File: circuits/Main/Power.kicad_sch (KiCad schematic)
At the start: 55 parts, among them IC1 DCDC_MPM3620A, J1 Conn_01x02_Male, J10 Conn_01x02_Male, J11 Conn_01x02_Male, J12 Conn_01x02_Male, J13 Conn_01x02_Male, J14 Conn_01x02_Male, J15 Conn_01x02_Male, J9 Conn_01x02_Male, Q1 DI035P04PT, Q2 BSS138, Q3 SSM3J332R, Q4 BSS138, Q5 DI035P04PT, SW1 SW_SPDT_White, U1 AZ1117CH-3.3

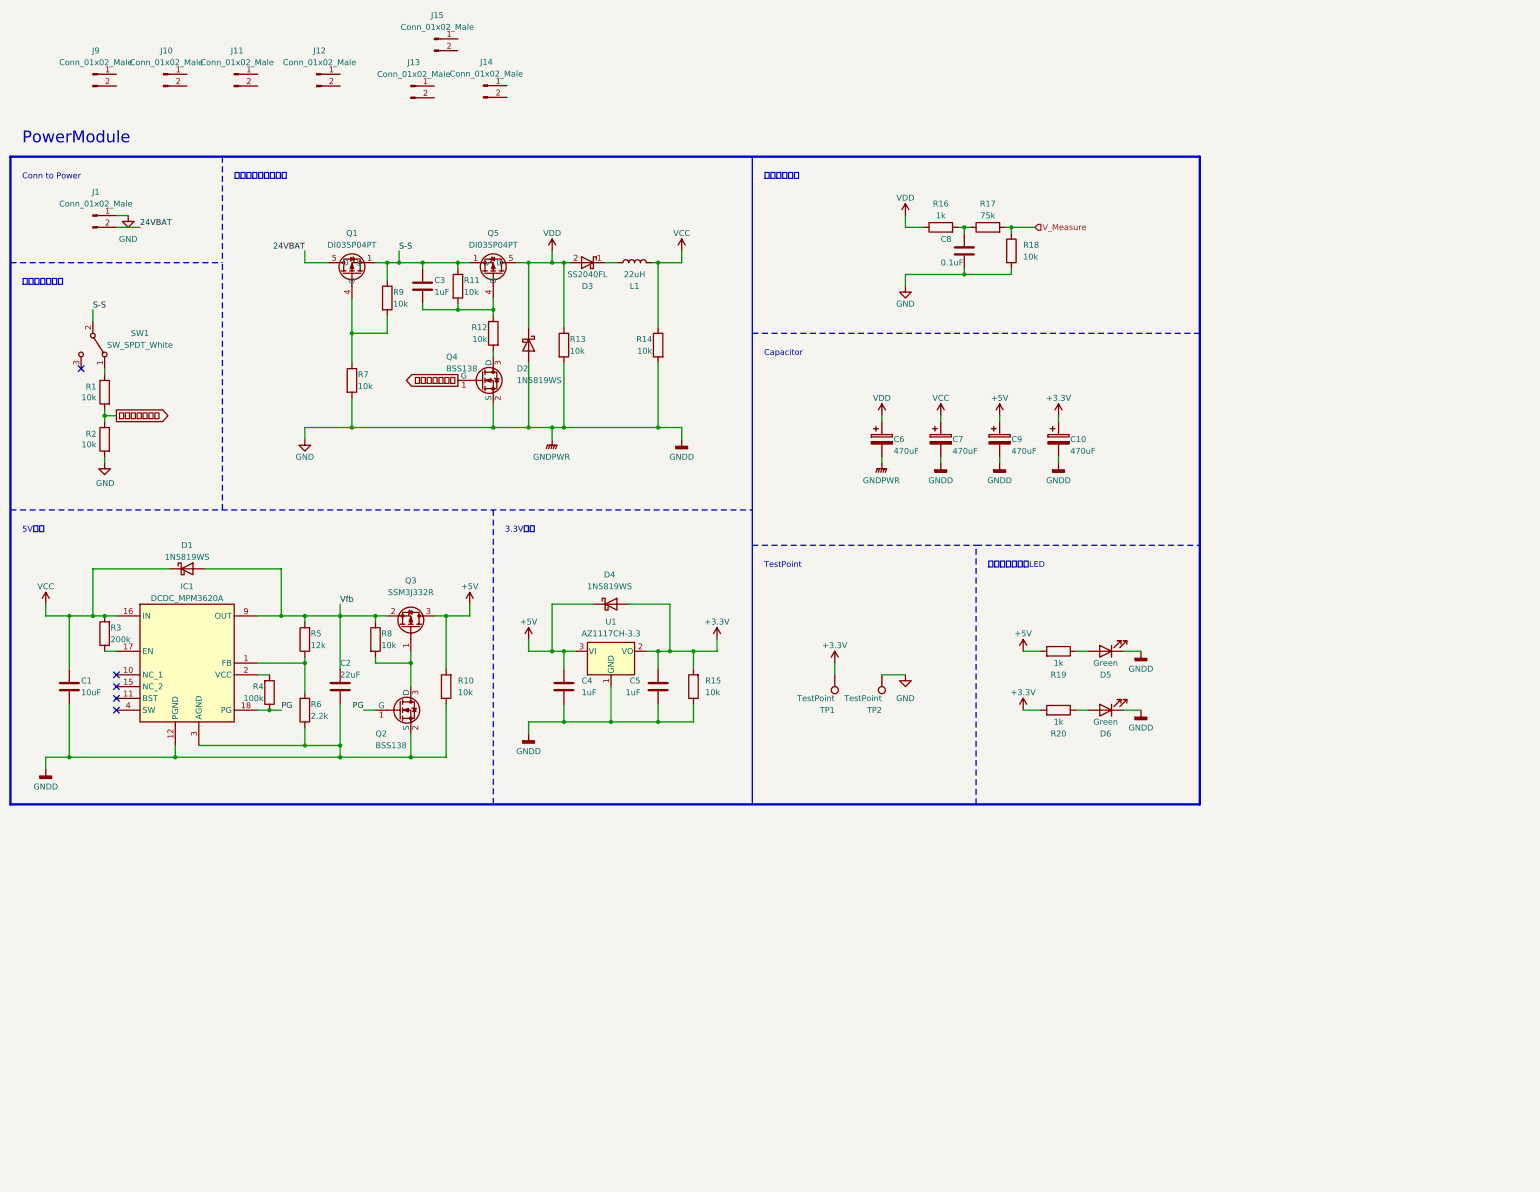
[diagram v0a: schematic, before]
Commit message: こみっと
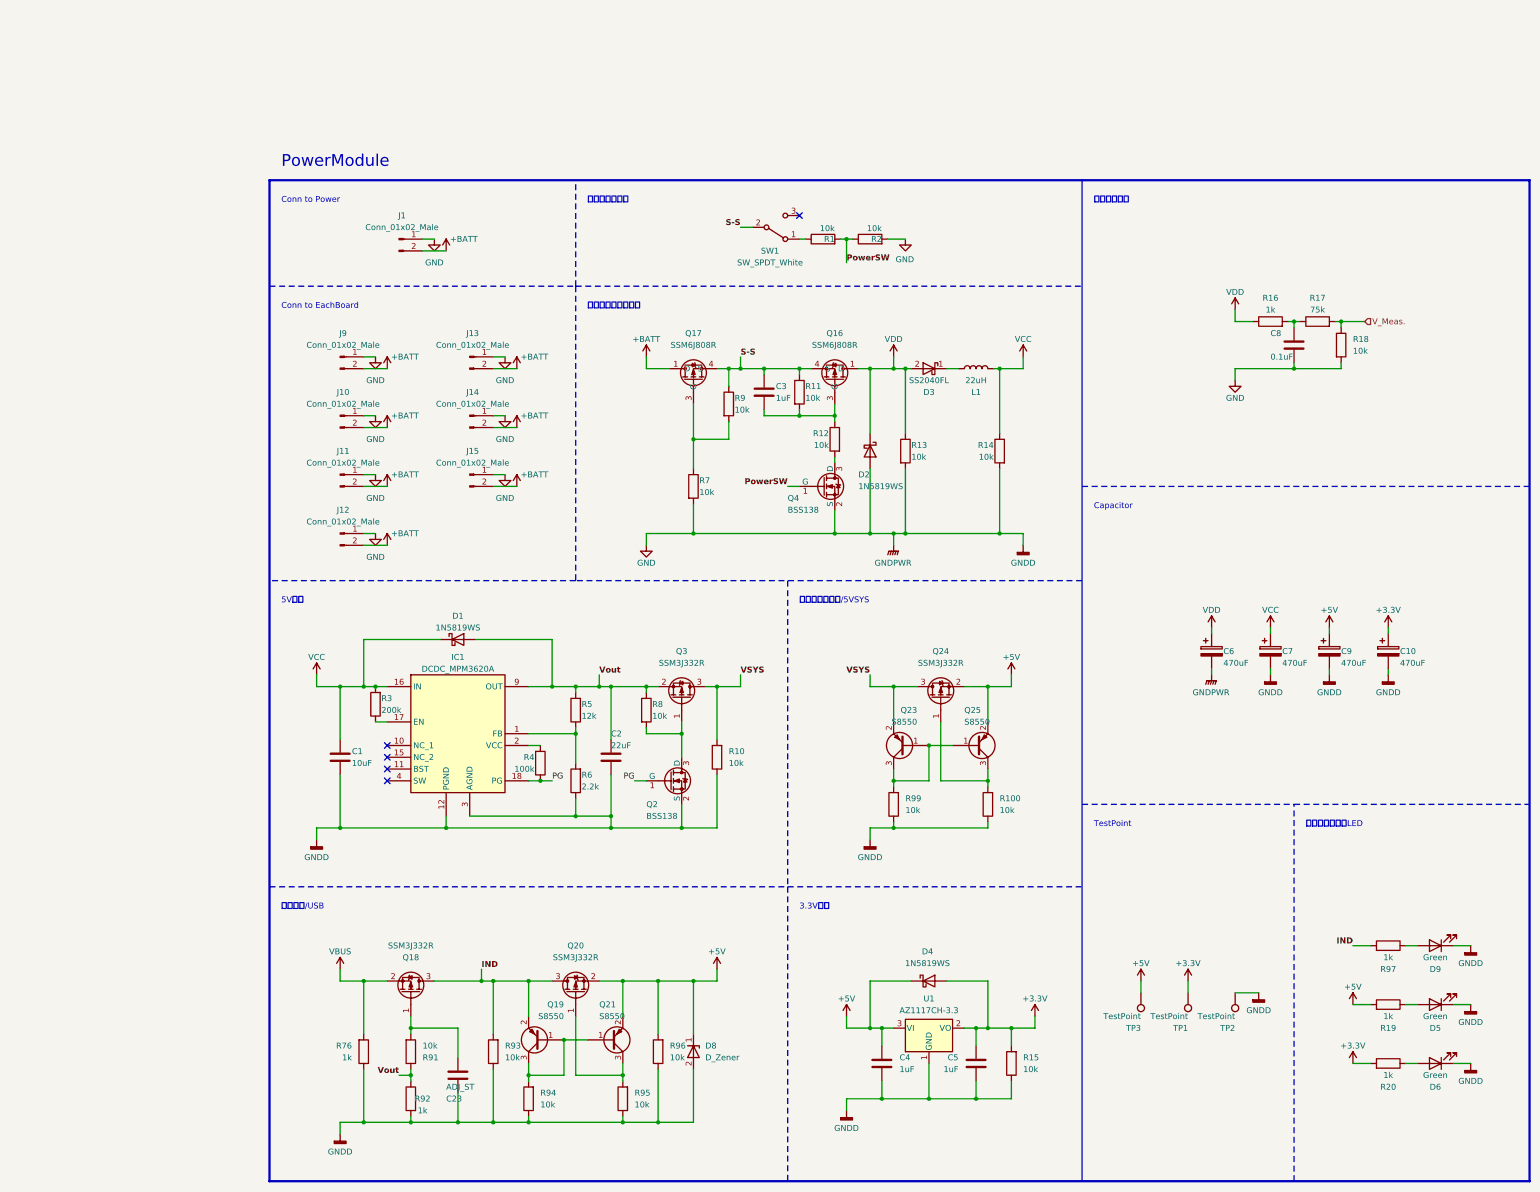
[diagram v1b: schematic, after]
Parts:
- removed Q1, Q5: DI035P04PT, MyLibrary:Package_TSON-Advance, symbol Transistor_FET:AON6411
- added C23: ADJ_ST, Capacitor_SMD:C_0603_1608Metric, symbol Device:C
- added D8: D_Zener, Diode_SMD:D_SOD-323_HandSoldering, symbol Device:D_Zener
- added D9: Green, LED_SMD:LED_0603_1608Metric_Pad1.05x0.95mm_HandSolder, symbol Device:LED
- added Q16, Q17: SSM6J808R, MyLibrary:Package_TSOP6F, symbol Transistor_FET:PMN48XP
- added Q18, Q20, Q24: SSM3J332R, Package_TO_SOT_SMD:SOT-23W, symbol Device:Q_PMOS_GSD
- added Q19, Q21, Q23, Q25: S8550, Package_TO_SOT_SMD:SOT-23, symbol Device:Q_PNP_BEC
- added R100, R91, R93, R94, R95, R96, R99: 10k, Resistor_SMD:R_0402_1005Metric, symbol Device:R
- added R76, R92, R97: 1k, Resistor_SMD:R_0402_1005Metric, symbol Device:R
- added TP3: TestPoint, TestPoint:TestPoint_THTPad_D2.0mm_Drill1.0mm, symbol Connector:TestPoint
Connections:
- net 24VBAT is gone; now on net +BATT: J1.2 (Pin_2)
- net +5V: now also D8.1 (K), Q20.2 (S), Q21.2 (E), Q24.2 (S), Q25.2 (E), R96.2, TP3.1; no longer Q3.3 (D), R10.2
- net GND: now also J10.1 (Pin_1), J11.1 (Pin_1), J12.1 (Pin_1), J13.1 (Pin_1), J14.1 (Pin_1), J15.1 (Pin_1), J9.1 (Pin_1), C23.1, D8.2 (A), D9.1 (K), R100.1, R76.1, R92.2, R93.1, R94.1, R95.1, R96.1, R99.1
- net S-S: now also Q16.4 (S), Q17.4 (S)
- net VDD: now also Q16.1 (D), Q16.2 (D), Q16.5 (D), Q16.6 (D)
- net at R7.1, R9.2: now also Q17.3 (G)
- net at C3.2, R11.2, R12.1: now also Q16.3 (G)
- net +BATT: now reaches J15.2 (Pin_2)
- net +BATT: now also J10.2 (Pin_2), J11.2 (Pin_2), J12.2 (Pin_2), J13.2 (Pin_2), J14.2 (Pin_2), J9.2 (Pin_2), Q17.1 (D), Q17.2 (D), Q17.5 (D), Q17.6 (D)
- net V_Measure renamed V_Meas.
- net Vfb renamed Vout
- net Vout: now also R91.1, R92.1
- net 主電源スイッチ renamed PowerSW
- new net: D9.2 (A), R97.1
- new net: Q19.1 (B), Q19.3 (C), Q21.1 (B), R94.2
- new net: Q23.1 (B), Q23.3 (C), Q25.1 (B), R99.2
- new net: C23.2, Q18.1 (G), R91.2
- new net: Q24.1 (G), Q25.3 (C), R100.2
- new net: Q20.1 (G), Q21.3 (C), R95.2
- new net IND: Q18.3 (D), Q19.2 (E), Q20.3 (D), R93.2, R97.2
- new net VBUS: Q18.2 (S), R76.2
- new net VSYS: Q23.2 (E), Q24.3 (D), Q3.3 (D), R10.2
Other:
- note added: "Conn to EachBoard"
- note added: "理想ダイオード/5VSYS"
- note added: "電源切替/USB"
- moved on the sheet: C1, C10, C2, C3, C4, C5, C6, C7, C8, C9, D1, D2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
